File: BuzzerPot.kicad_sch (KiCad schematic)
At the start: 9 parts, among them J1 ConnM_01x03_Horizontal_2.54mm, U1 SC8002B

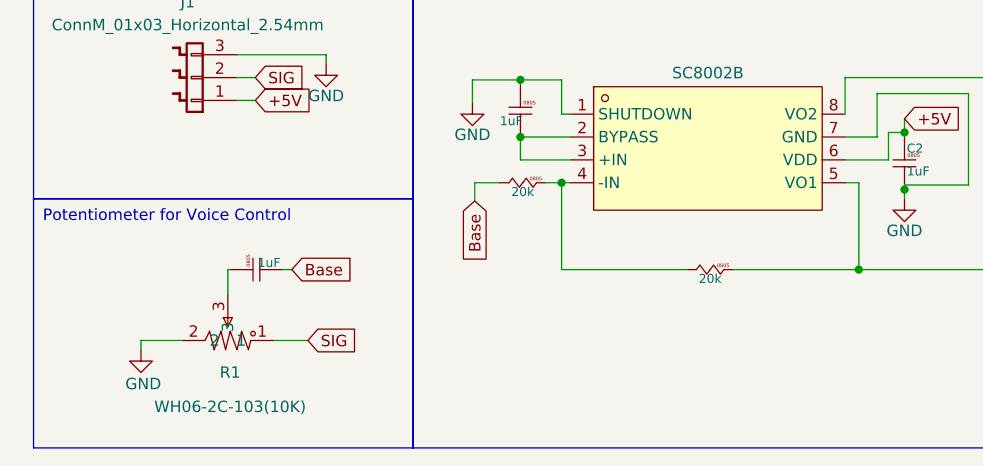
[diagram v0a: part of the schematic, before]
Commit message: Updated Version 2
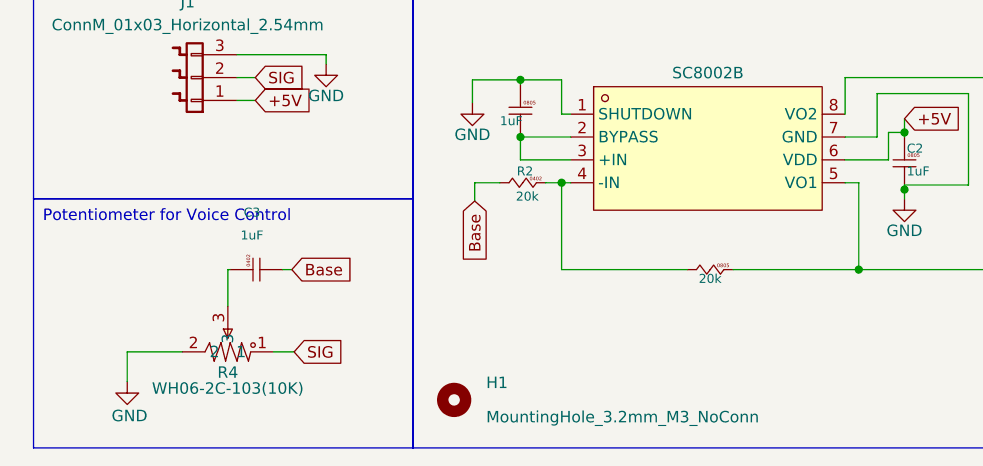
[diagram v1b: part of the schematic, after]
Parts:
- removed C3: 1uF, Remal_KiCadLib:C_0805_2012m, symbol Remal_KiCadLib:C_0805_2012m
- removed R1: WH06-2C-103(10K), easyeda2kicad:RES-ADJ-TH_WH06-2C-103, symbol easyeda2kicad:WH06-2C-103(10K)
- removed R2: 20k, Remal_KiCadLib:R_0805_2012m, symbol Remal_KiCadLib:R_0805_2012m
- added C3: 1uF, Remal_KiCadLib:C_0402_1005m, symbol Remal_KiCadLib:C_0402_1005m
- added H1: MountingHole_3.2mm_M3_NoConn, Remal_KiCadLib:MountingHole_3.2mm_M3_NoConn, symbol Remal_KiCadLib:MountingHole_3.2mm_M3_NoConn
- added R2: 20k, Remal_KiCadLib:R_0402_1005m, symbol Remal_KiCadLib:R_0402_1005m
- added R4: WH06-2C-103(10K), easyeda2kicad:RES-ADJ-TH_WH06-2C-103, symbol easyeda2kicad:WH06-2C-103(10K)
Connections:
- net Base: now also C3.2, R2.1
- net GND: now also R4.2
- net SIG: now also R4.1
- net at R3.1, U1.4 (-IN): now also R2.2
- new net: C3.1, R4.3
